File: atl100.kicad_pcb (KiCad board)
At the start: 2 copper layers, 150 x 100 mm, 43 parts, among them J1 Conn_01x04_Pin, J2 Screw_Terminal_01x02, J3 Screw_Terminal_01x02, J4 Screw_Terminal_01x02, J5 Screw_Terminal_01x02, J6 Screw_Terminal_01x04, J7 Screw_Terminal_01x04, J8 Screw_Terminal_01x06, U2 ESP32-S3 DevKit, U3 HW-519, U4 ADS1115 Module, U6 SIM7070G Module

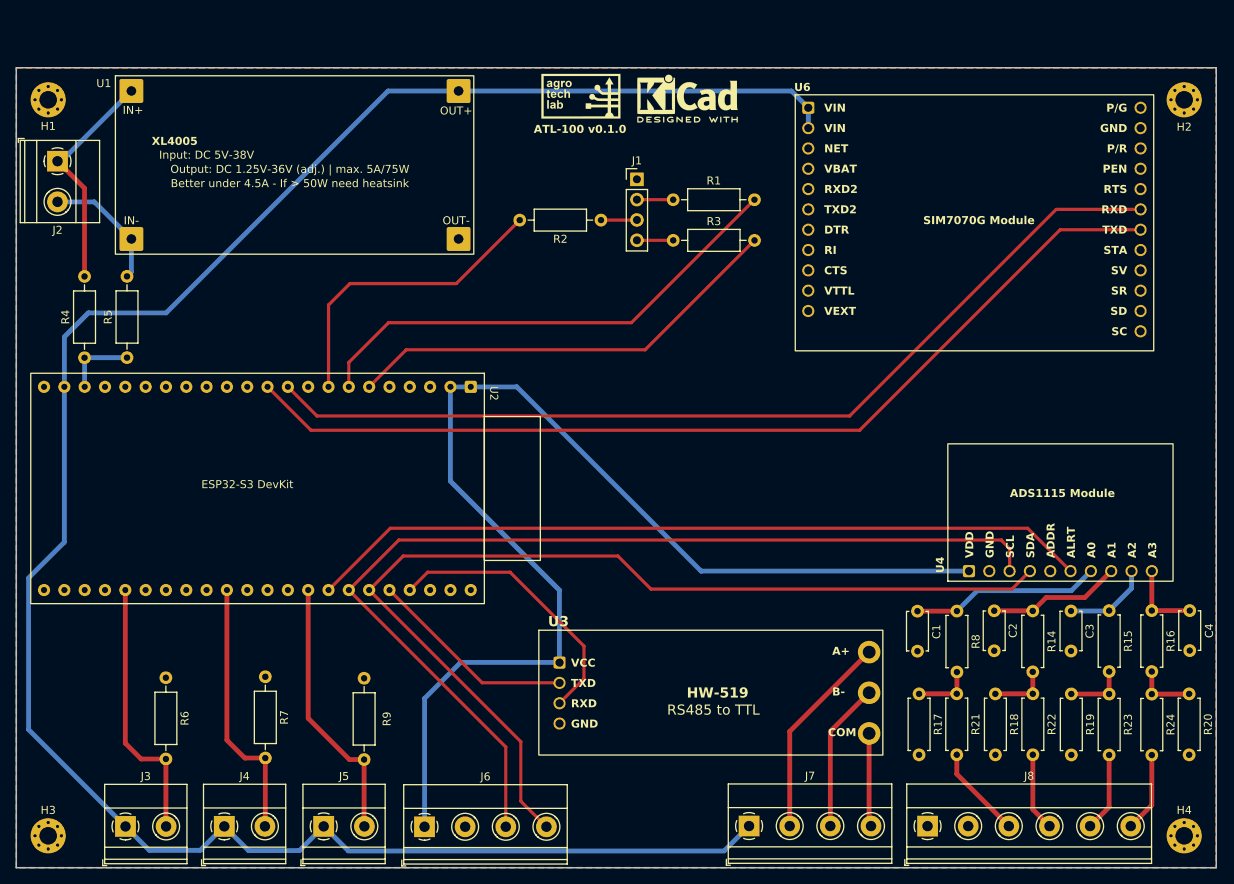
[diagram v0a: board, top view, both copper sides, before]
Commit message: feat: Updated to v0.2.0
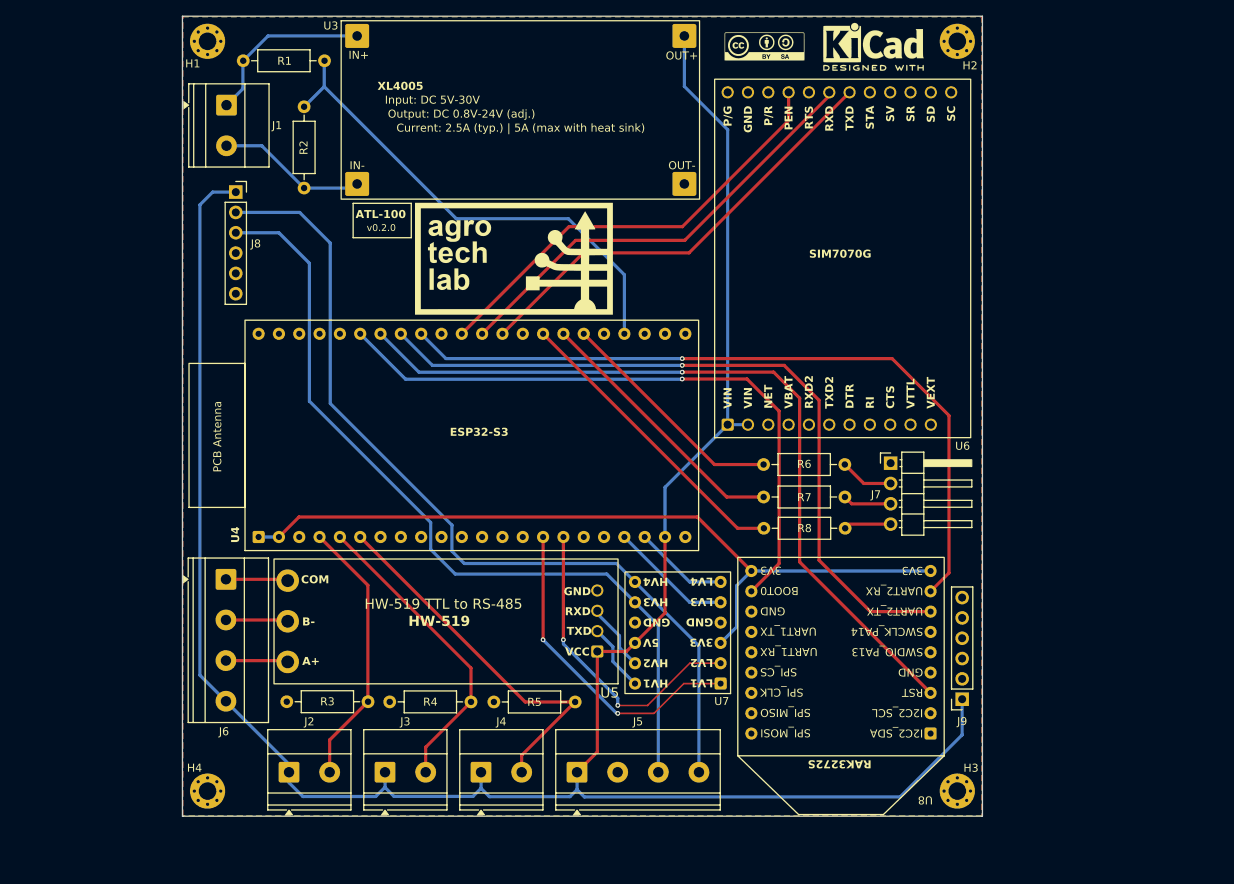
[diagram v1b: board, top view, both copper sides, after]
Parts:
- removed C1, C2, C3, C4: 100nF, Capacitor_THT:C_Disc_D4.7mm_W2.5mm_P5.00mm
- removed G***: LOGO, LOGO
- removed R14, R15, R16: 3k3, Resistor_THT:R_Axial_DIN0207_L6.3mm_D2.5mm_P7.62mm_Horizontal
- removed R17, R18, R19, R20: 100R, Resistor_THT:R_Axial_DIN0207_L6.3mm_D2.5mm_P7.62mm_Horizontal
- removed R21, R22, R23, R24: 50R, Resistor_THT:R_Axial_DIN0207_L6.3mm_D2.5mm_P7.62mm_Horizontal
- removed R9: 10k, Resistor_THT:R_Axial_DIN0207_L6.3mm_D2.5mm_P10.16mm_Horizontal
- removed REF**: KiCad-Logo2_5mm_SilkScreen, Symbol:KiCad-Logo2_5mm_SilkScreen
- removed U1: ~, AgroTechLab:XL4005_Module
- removed U2: ESP32-S3 DevKit, AgroTechLab:ESP32S3N16R8_DevKit
- added J9: Conn_01x06_Socket, Connector_PinSocket_2.54mm:PinSocket_1x06_P2.54mm_Vertical, F.Cu at (188.7, 126.2)
- added U5: HW-519, AgroTechLab:HW-519, F.Cu at (143.1, 120.2)
- added U7: Logical Level Converter, AgroTechLab:Logical Level Converter, F.Cu at (158.5, 124.2)
- added U8: RAK3272S, AgroTechLab:RAK3272S, F.Cu at (184.7, 130.5)
- added agrotechlab_logo: Logo AgroTechLab, AgroTechLab:Logo AgroTechLab, F.Cu at (132.6, 71.2)
- added cc_by_sa_logo: Logo CC-BY-SA, AgroTechLab:Logo CC-BY-SA, F.Cu at (164.0, 44.6)
- added kicad_logo: KiCad-Logo2_5mm_SilkScreen, Symbol:KiCad-Logo2_5mm_SilkScreen, F.Cu at (177.6, 44.6)
- J1: value Conn_01x04_Pin -> Screw_Terminal_01x02; footprint Connector_PinHeader_2.54mm:PinHeader_1x04_P2.54mm_Vertical -> TerminalBlock_Phoenix:TerminalBlock_Phoenix_MKDS-1,5-2-5.08_1x02_P5.08mm_Horizontal
- J5: value Screw_Terminal_01x02 -> Screw_Terminal_01x04; footprint TerminalBlock_Phoenix:TerminalBlock_Phoenix_MKDS-1,5-2-5.08_1x02_P5.08mm_Horizontal -> TerminalBlock_Phoenix:TerminalBlock_Phoenix_MKDS-1,5-4-5.08_1x04_P5.08mm_Horizontal
- J7: value Screw_Terminal_01x04 -> Conn_01x04_Pin; footprint TerminalBlock_Phoenix:TerminalBlock_Phoenix_MKDS-1,5-4-5.08_1x04_P5.08mm_Horizontal -> Connector_PinHeader_2.54mm:PinHeader_1x04_P2.54mm_Horizontal
- J8: value Screw_Terminal_01x06 -> Conn_01x06_Socket; footprint TerminalBlock_Phoenix:TerminalBlock_Phoenix_MKDS-1,5-6-5.08_1x06_P5.08mm_Horizontal -> Connector_PinSocket_2.54mm:PinSocket_1x06_P2.54mm_Vertical
- R1: value 67R -> 8k
- R2: value 42R -> 1k
- R3: value 17R -> 4.7k
- R5: value 1.2k -> 10k
- R6: value 4.7k -> 17R
- R7: value 10k -> 42R
- R8: value 3k3 -> 67R; footprint Resistor_THT:R_Axial_DIN0207_L6.3mm_D2.5mm_P7.62mm_Horizontal -> Resistor_THT:R_Axial_DIN0207_L6.3mm_D2.5mm_P10.16mm_Horizontal
- U3: value HW-519 -> XL4005; footprint AgroTechLab:HW-519 -> AgroTechLab:XL4005
- U4: value ADS1115 Module -> ESP32-S3; footprint AgroTechLab:ADS1115 Module -> AgroTechLab:ESP32-S3 N16R8
- U6: value SIM7070G Module -> SIM7070G; footprint AgroTechLab:SIM7070G Module -> AgroTechLab:SIM7070G
- moved H4 122.2 mm to (94.3, 137.7)
- moved J8 117.3 mm to (97.9, 62.8)
- moved H3 113.8 mm to (188.1, 137.7)
- moved R6 89.0 mm to (174.0, 96.9), turned to 180 degrees
- moved U4 88.9 mm to (100.7, 105.9)
- moved U3 82.3 mm to (113.0, 43.3)
- moved J2 81.7 mm to (104.5, 135.3), turned to 0 degrees
- moved R7 75.9 mm to (174.0, 100.9), turned to 180 degrees
- moved R3 75.2 mm to (104.2, 126.5)
- moved R5 70.6 mm to (140.3, 126.5), turned to 180 degrees
- moved R4 57.5 mm to (117.1, 126.5), turned to 0 degrees
- moved J1 52.1 mm to (96.7, 51.9), turned to -90 degrees
- moved J7 48.7 mm to (179.7, 96.7)
- moved R1 46.9 mm to (109.0, 46.4), turned to 180 degrees
- moved U6 40.9 mm to (159.4, 91.9), turned to 90 degrees
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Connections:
- J1 pad 1: GND -> PWR_IN+
- J1 pad 2: Net-(J1-Pin_2) -> PWR_IN-
- J2 pad 1: PWR_IN+ -> +5V
- J2 pad 2: PWR_IN- -> WS-
- J3 pad 2: WS- -> AN-
- J4 pad 2: AN- -> PL-
- J5 pad 2: PL- -> GND
- J6 pad 1: +3V3 -> RS485_COM
- J6 pad 2: GND -> RS485_B-
- J6 pad 3: I2C_SCL -> RS485_A+
- J6 pad 4: I2C_SDA -> +5V
- J7 pad 1: +5V -> GND
- J7 pad 2: RS485_A+ -> Net-(J7-Pin_2)
- J7 pad 3: RS485_B- -> Net-(J7-Pin_3)
- J7 pad 4: RS485_COM -> Net-(J7-Pin_4)
- J8 pad 1: GND -> +5V
- J8 pad 2: unconnected-(J8-Pin_2-Pad2) -> I2C_SCL_5V
- J8 pad 3: AI1 -> I2C_SDA_5V
- J8 pad 4: AI2 -> unconnected-(J8-Pin_4-Pad4)
- J8 pad 5: AI3 -> unconnected-(J8-Pin_5-Pad5)
- J8 pad 6: AI4 -> GND
- R1 pad 1: Net-(J1-Pin_2) -> PWR_SENSOR
- R1 pad 2: LED_RED -> PWR_IN+
- R2 pad 1: Net-(J1-Pin_3) -> PWR_SENSOR
- R2 pad 2: LED_GREEN -> PWR_IN-
- R3 pad 1: Net-(J1-Pin_4) -> GND
- R3 pad 2: LED_BLUE -> WS-
- R4 pad 1: PWR_SENSOR -> GND
- R4 pad 2: PWR_IN+ -> AN-
- R5 pad 1: PWR_SENSOR -> PL-
- R5 pad 2: PWR_IN- -> GND
- R6 pad 1: GND -> Net-(J7-Pin_2)
- R6 pad 2: WS- -> LED_BLUE
- R7 pad 1: GND -> Net-(J7-Pin_3)
- R7 pad 2: AN- -> LED_GREEN
- R8 pad 1: Net-(U4-A0) -> Net-(J7-Pin_4)
- R8 pad 2: Net-(R17-Pad1) -> LED_RED
- U3 pad 1: +3V3 -> PWR_IN+
- U3 pad 2: MCU_RXD - RS485_TXD -> PWR_IN-
- U3 pad 3: MCU_TXD - RS485_RXD -> +5V
- U4 pad 10: Net-(U4-A3) -> unconnected-(U4-GPIO17/RTC_GPIO17/ADC2_CH6/U1TXD-Pad10)
- U4 pad 2: GND -> +3V3
- U4 pad 3: I2C_SCL -> unconnected-(U4-RST-Pad3)
- U4 pad 4: I2C_SDA -> WS-
- U4 pad 5: GND -> AN-
- U4 pad 6: ADC_ALERT -> PL-
- U4 pad 7: Net-(U4-A0) -> unconnected-(U4-GPIO7/RTC_GPIO7/ADC1_CH6-Pad7)
- U4 pad 8: Net-(U4-A1) -> unconnected-(U4-GPIO15/RTC_GPIO15/ADC2_CH4/U0RTS-Pad8)
- U4 pad 9: Net-(U4-A2) -> unconnected-(U4-GPIO16/RTC_GPIO16/ADC2_CH5/U0CTS-Pad9)
- U6 pad 12: unconnected-(U6-P/G-Pad12) -> GND
- U6 pad 15: unconnected-(U6-PEN-Pad15) -> LTE_PEN
- U6 pad 17: MCU_TXD - LTE_RXD -> LTE_RX
- U6 pad 18: MCU_RXD - LTE_TXD -> LTE_TX
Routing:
- net I2C_SCL: track 126.2 -> 0.00 mm
- net I2C_SDA: track 125.8 -> 0.00 mm
- net MCU_RXD - LTE_TXD: track 121.8 -> 0.00 mm
- net MCU_TXD - LTE_RXD: track 118.8 -> 0.00 mm
- net I2C_SCL_5V: track 0.00 -> 109.8 mm
- net I2C_SDA_5V: track 0.00 -> 103.6 mm
- net LORA_RST: track 0.00 -> 99.5 mm, vias 0 -> 1
- net ADC_ALERT: track 98.2 -> 0.00 mm
- net LORA_RX: track 0.00 -> 93.1 mm, vias 0 -> 1
- net LORA_TX: track 0.00 -> 92.4 mm, vias 0 -> 1
- net LORA_BOOT0: track 0.00 -> 80.3 mm, vias 0 -> 1
- net LTE_RX: track 0.00 -> 56.2 mm
- net LTE_TX: track 0.00 -> 55.9 mm
- net LTE_PEN: track 0.00 -> 55.4 mm
- net PWR_SENSOR: track 8.96 -> 61.4 mm
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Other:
- board size 150 x 100 mm -> 100 x 100 mm
- board text added: "ATL-100"
- board text added: "v0.2.0"
- board text removed: "ATL-100 v0.1.0"
